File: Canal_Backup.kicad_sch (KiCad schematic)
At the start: 0 parts

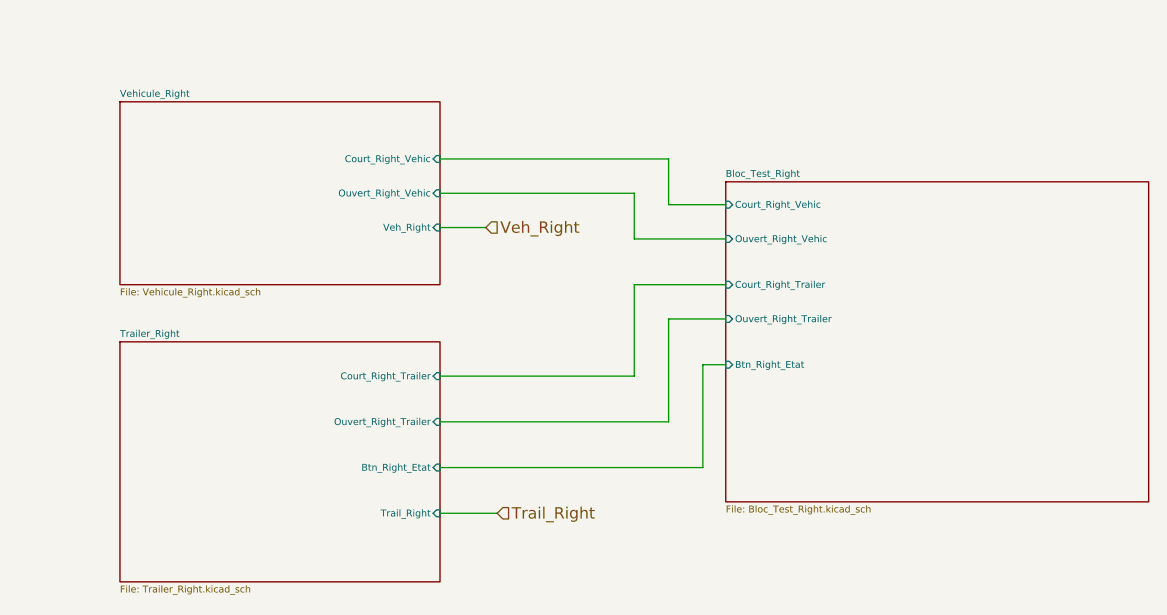
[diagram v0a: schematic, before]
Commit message: Add files via upload
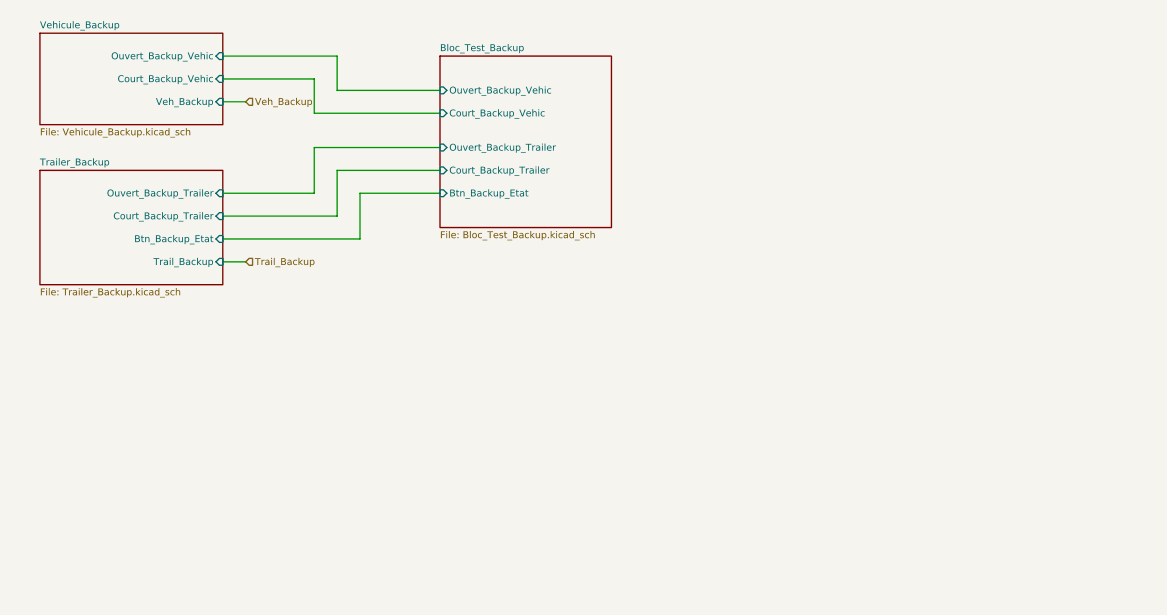
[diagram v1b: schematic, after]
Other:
- removed sheet Bloc_Test_Right
- removed sheet Trailer_Right
- removed sheet Vehicule_Right
- added sheet Bloc_Test_Backup (Bloc_Test_Backup.kicad_sch)
- added sheet Trailer_Backup (Trailer_Backup.kicad_sch)
- added sheet Vehicule_Backup (Vehicule_Backup.kicad_sch)

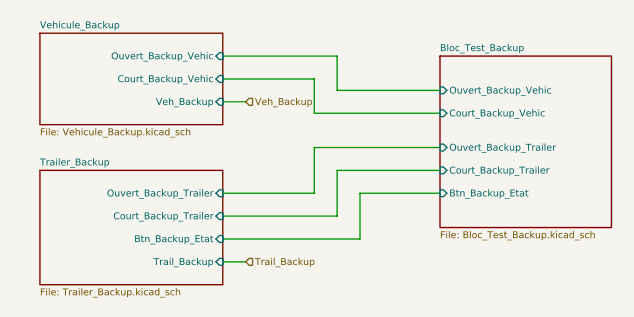
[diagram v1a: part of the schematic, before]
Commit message: Add files via upload
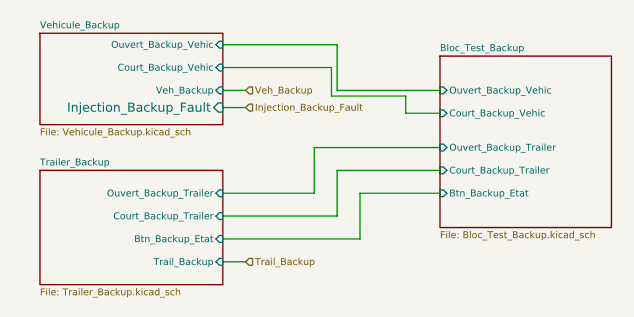
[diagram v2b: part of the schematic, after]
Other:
- sheet Vehicule_Backup ports: added Injection_Backup_Fault; removed none
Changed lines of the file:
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@@
 	(wire
 		(pts
-			(xy 39.37 30.48) (xy 41.91 30.48)
+			(xy 39.37 29.21) (xy 41.91 29.21)
 		)
 		(stroke
@@
 	(wire
 		(pts
-			(xy 39.37 27.94) (xy 49.53 27.94)
+			(xy 41.91 31.115) (xy 39.37 31.115)
 		)
 		(stroke
@@
 	(wire
 		(pts
+			(xy 59.69 31.75) (xy 63.5 31.75)
+		)
+		(stroke
+			(width 0)
+			(type default)
+		)
+	)
+	(wire
+		(pts
 			(xy 52.07 29.21) (xy 63.5 29.21)
 		)
@@
 	(wire
 		(pts
-			(xy 52.07 25.4) (xy 52.07 29.21)
+			(xy 52.07 24.13) (xy 52.07 29.21)
 		)
 		(stroke
@@
 	(wire
 		(pts
-			(xy 49.53 27.94) (xy 49.53 31.75)
-		)
-		(stroke
-			(width 0)
-			(type default)
-		)
-	)
-	(wire
-		(pts
-			(xy 39.37 25.4) (xy 52.07 25.4)
+			(xy 39.37 24.13) (xy 52.07 24.13)
 		)
 		(stroke
@@
 	(wire
 		(pts
-			(xy 49.53 31.75) (xy 63.5 31.75)
+			(xy 51.435 29.845) (xy 59.69 29.845)
+		)
+		(stroke
+			(width 0)
+			(type default)
+		)
+	)
+	(wire
+		(pts
+			(xy 39.37 26.67) (xy 51.435 26.67)
+		)
+		(stroke
+			(width 0)
+			(type default)
+		)
+	)
+	(wire
+		(pts
+			(xy 59.69 29.845) (xy 59.69 31.75)
+		)
+		(stroke
+			(width 0)
+			(type default)
+		)
+	)
+	(wire
+		(pts
+			(xy 51.435 26.67) (xy 51.435 29.845)
 		)
 		(stroke
@@
 		)
 	)
+	(hierarchical_label "Injection_Backup_Fault"
+		(shape input)
+		(at 41.91 31.115 0)
+		(effects
+			(font
+				(size 0.762 0.762)
+			)
+			(justify left)
+		)
+	)
 	(hierarchical_label "Veh_Backup"
 		(shape input)
-		(at 41.91 30.48 0)
+		(at 41.91 29.21 0)
 		(effects
 			(font
@@
 		)
 		(pin "Court_Backup_Vehic" input
-			(at 39.37 27.94 0)
+			(at 39.37 26.67 0)
 			(effects
 				(font
@@
 		)
 		(pin "Ouvert_Backup_Vehic" input
-			(at 39.37 25.4 0)
+			(at 39.37 24.13 0)
 			(effects
 				(font
@@
 		)
 		(pin "Veh_Backup" input
-			(at 39.37 30.48 0)
-			(effects
-				(font
-					(size 0.762 0.762)
-				)
-				(justify right)
+			(at 39.37 29.21 0)
+			(effects
+				(font
+					(size 0.762 0.762)
+				)
+				(justify right)
+			)
+		)
+		(pin "Injection_Backup_Fault" input
+			(at 39.37 31.115 0)
+			(effects
+				(font
+					(size 1.016 1.016)
+				)
+				(justify right)

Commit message: Add files via upload
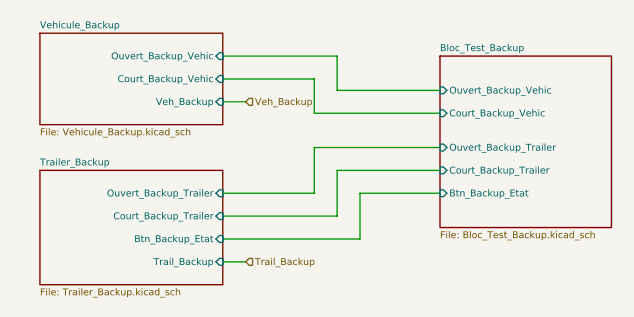
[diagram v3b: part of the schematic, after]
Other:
- sheet Vehicule_Backup ports: added none; removed Injection_Backup_Fault
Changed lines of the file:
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@@
 	(wire
 		(pts
-			(xy 39.37 29.21) (xy 41.91 29.21)
+			(xy 39.37 30.48) (xy 41.91 30.48)
 		)
 		(stroke
@@
 	(wire
 		(pts
-			(xy 41.91 31.115) (xy 39.37 31.115)
+			(xy 39.37 27.94) (xy 49.53 27.94)
 		)
 		(stroke
@@
 	(wire
 		(pts
-			(xy 59.69 31.75) (xy 63.5 31.75)
-		)
-		(stroke
-			(width 0)
-			(type default)
-		)
-	)
-	(wire
-		(pts
 			(xy 52.07 29.21) (xy 63.5 29.21)
 		)
@@
 	(wire
 		(pts
-			(xy 52.07 24.13) (xy 52.07 29.21)
+			(xy 52.07 25.4) (xy 52.07 29.21)
 		)
 		(stroke
@@
 	(wire
 		(pts
-			(xy 39.37 24.13) (xy 52.07 24.13)
+			(xy 49.53 27.94) (xy 49.53 31.75)
+		)
+		(stroke
+			(width 0)
+			(type default)
+		)
+	)
+	(wire
+		(pts
+			(xy 39.37 25.4) (xy 52.07 25.4)
 		)
 		(stroke
@@
 	(wire
 		(pts
-			(xy 51.435 29.845) (xy 59.69 29.845)
-		)
-		(stroke
-			(width 0)
-			(type default)
-		)
-	)
-	(wire
-		(pts
-			(xy 39.37 26.67) (xy 51.435 26.67)
-		)
-		(stroke
-			(width 0)
-			(type default)
-		)
-	)
-	(wire
-		(pts
-			(xy 59.69 29.845) (xy 59.69 31.75)
-		)
-		(stroke
-			(width 0)
-			(type default)
-		)
-	)
-	(wire
-		(pts
-			(xy 51.435 26.67) (xy 51.435 29.845)
+			(xy 49.53 31.75) (xy 63.5 31.75)
 		)
 		(stroke
@@
 		)
 	)
-	(hierarchical_label "Injection_Backup_Fault"
-		(shape input)
-		(at 41.91 31.115 0)
-		(effects
-			(font
-				(size 0.762 0.762)
-			)
-			(justify left)
-		)
-	)
 	(hierarchical_label "Veh_Backup"
 		(shape input)
-		(at 41.91 29.21 0)
+		(at 41.91 30.48 0)
 		(effects
 			(font
@@
 		)
 		(pin "Court_Backup_Vehic" input
-			(at 39.37 26.67 0)
+			(at 39.37 27.94 0)
 			(effects
 				(font
@@
 		)
 		(pin "Ouvert_Backup_Vehic" input
-			(at 39.37 24.13 0)
+			(at 39.37 25.4 0)
 			(effects
 				(font
@@
 		)
 		(pin "Veh_Backup" input
-			(at 39.37 29.21 0)
-			(effects
-				(font
-					(size 0.762 0.762)
-				)
-				(justify right)
-			)
-		)
-		(pin "Injection_Backup_Fault" input
-			(at 39.37 31.115 0)
-			(effects
-				(font
-					(size 1.016 1.016)
-				)
-				(justify right)
+			(at 39.37 30.48 0)
+			(effects
+				(font
+					(size 0.762 0.762)
+				)
+				(justify right)
